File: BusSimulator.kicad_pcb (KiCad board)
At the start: 2 copper layers, 15 parts, among them U1 MPM3620, U2 MPM3620

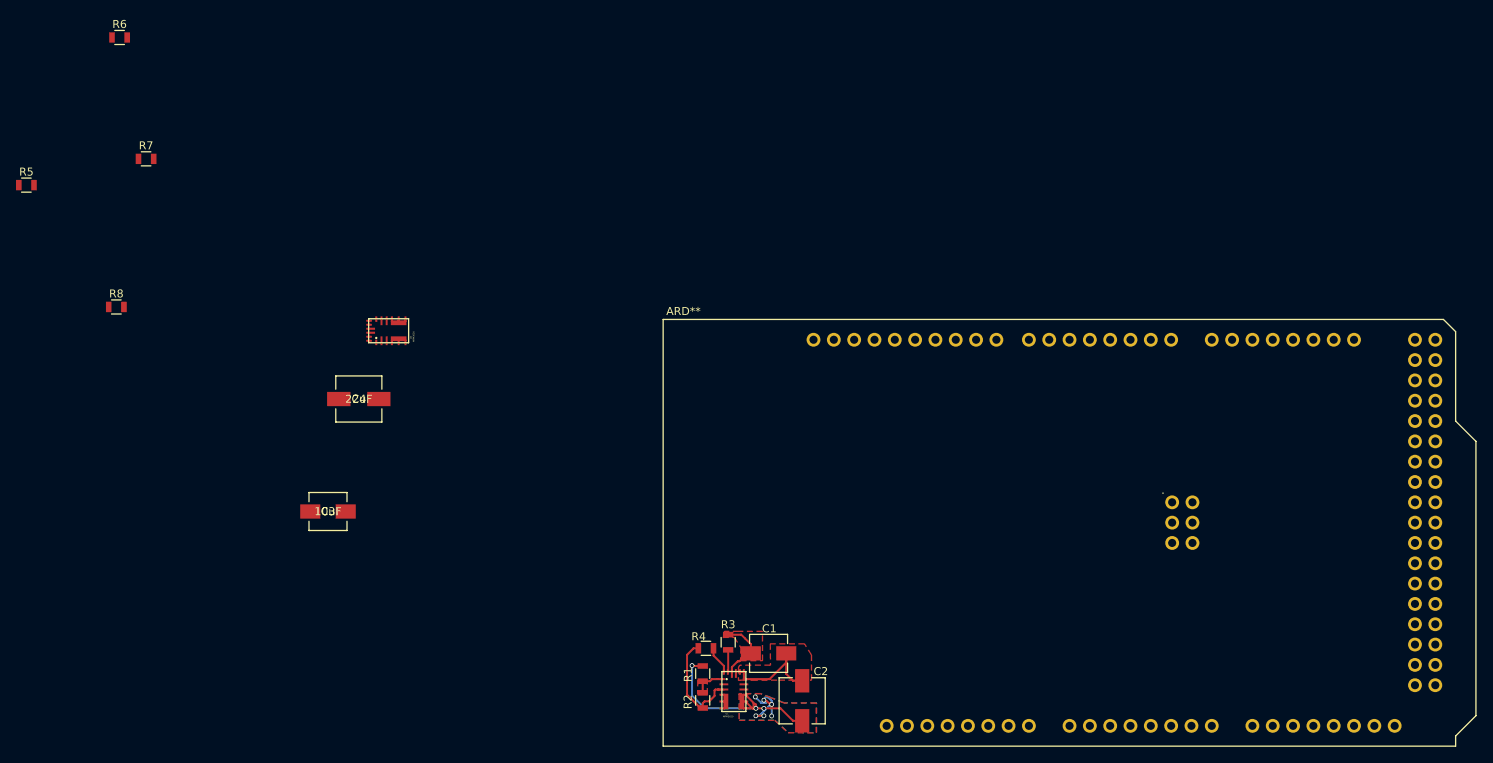
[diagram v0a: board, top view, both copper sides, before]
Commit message: Finished 3v3 and 5V
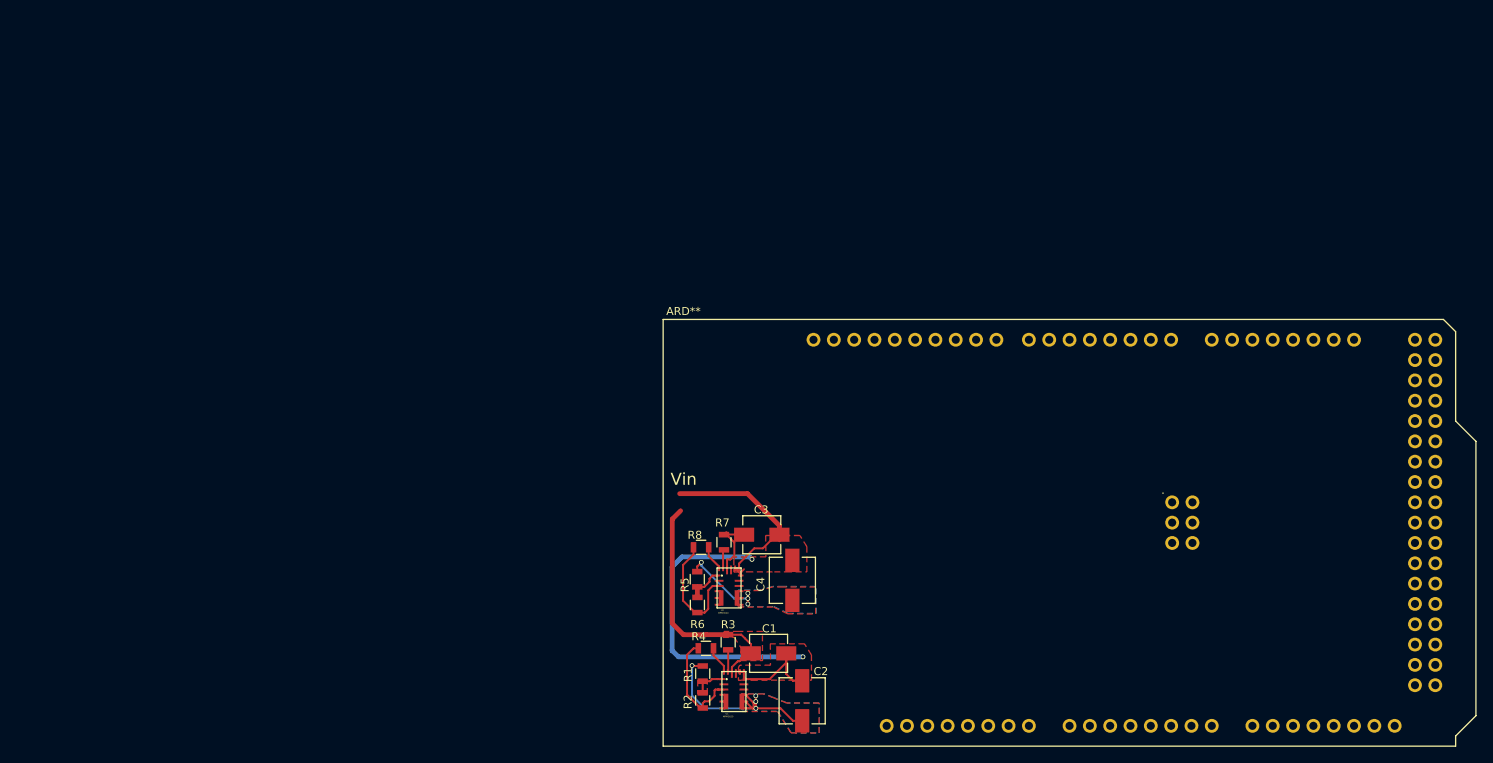
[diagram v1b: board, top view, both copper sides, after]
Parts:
- moved R6 101.2 mm to (114.3, 123.9), turned to 270 degrees
- moved R5 97.3 mm to (114.3, 120.7), turned to 270 degrees
- moved R7 86.7 mm to (117.6, 116.1), turned to 270 degrees
- moved R8 79.0 mm to (114.8, 116.7), turned to 180 degrees
- moved C4 58.7 mm to (126.2, 120.9), turned to 270 degrees
- moved C3 54.3 mm to (122.3, 115.2), turned to 180 degrees
- moved U2 53.3 mm to (118.2, 121.8), turned to 0 degrees
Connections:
- C3 pad 1: Earth -> GNDREF
- C4 pad 1: Earth -> GNDREF
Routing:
- net (no net): track 9.47 -> 37.8 mm, vias 6 -> 2
- net GNDREF: track 13.5 -> 39.7 mm
- net Net-(C1-Pad2): track 8.35 -> 30.4 mm
- net GNDA: track 13.9 -> 29.0 mm
- net +3V3: track 0.00 -> 10.7 mm, vias 0 -> 4
- net Net-(C3-Pad2): track 0.00 -> 8.35 mm
- net Net-(R5-Pad2): track 0.00 -> 4.66 mm
- net Net-(R8-Pad1): track 0.00 -> 3.17 mm
- net Net-(R7-Pad2): track 0.00 -> 2.36 mm
- net +5V: track 25.3 -> 26.9 mm, vias 3 -> 4
- added copper zone on B.Cu, net +3V3
- added copper zone on F.Cu, net +3V3
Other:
- board text added: "Vin"
